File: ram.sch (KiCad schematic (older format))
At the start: 7 parts, among them U1 LFE5U-85F-6BG381C

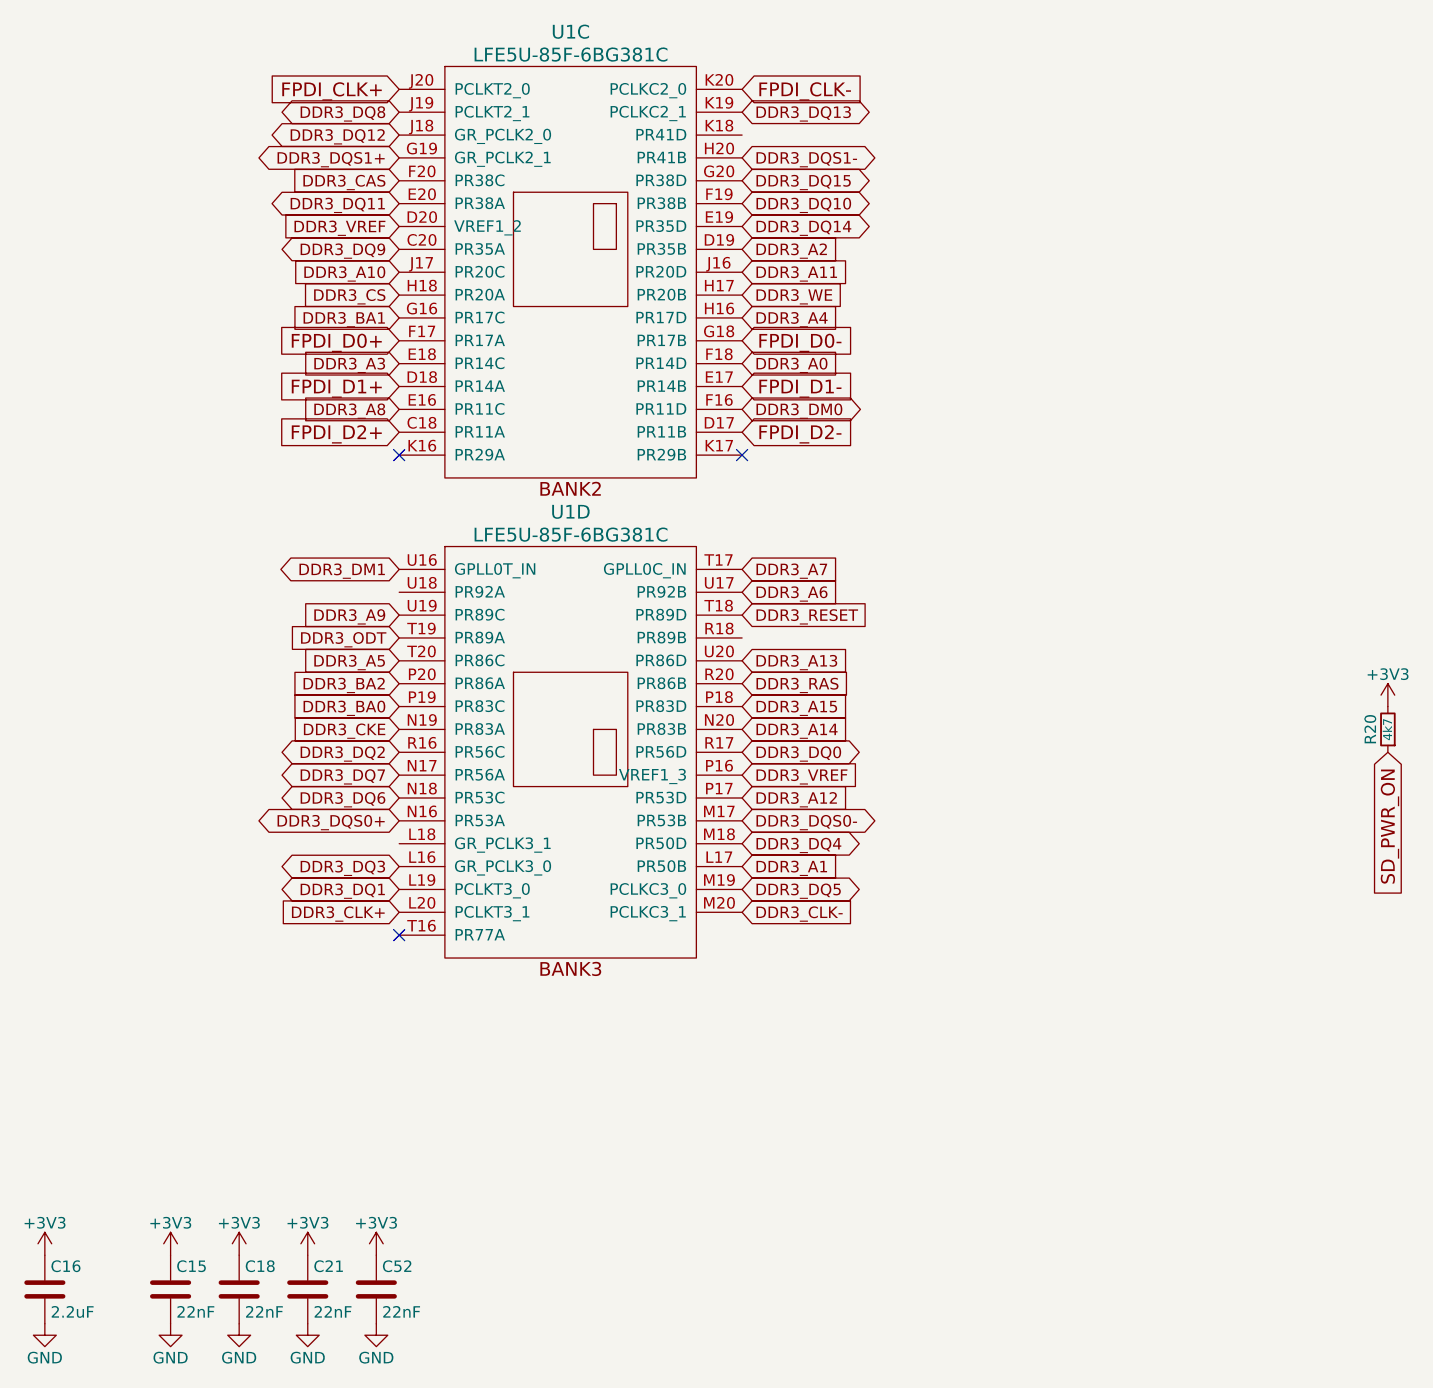
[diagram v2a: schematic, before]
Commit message: Adding SDRAM removind DDR3
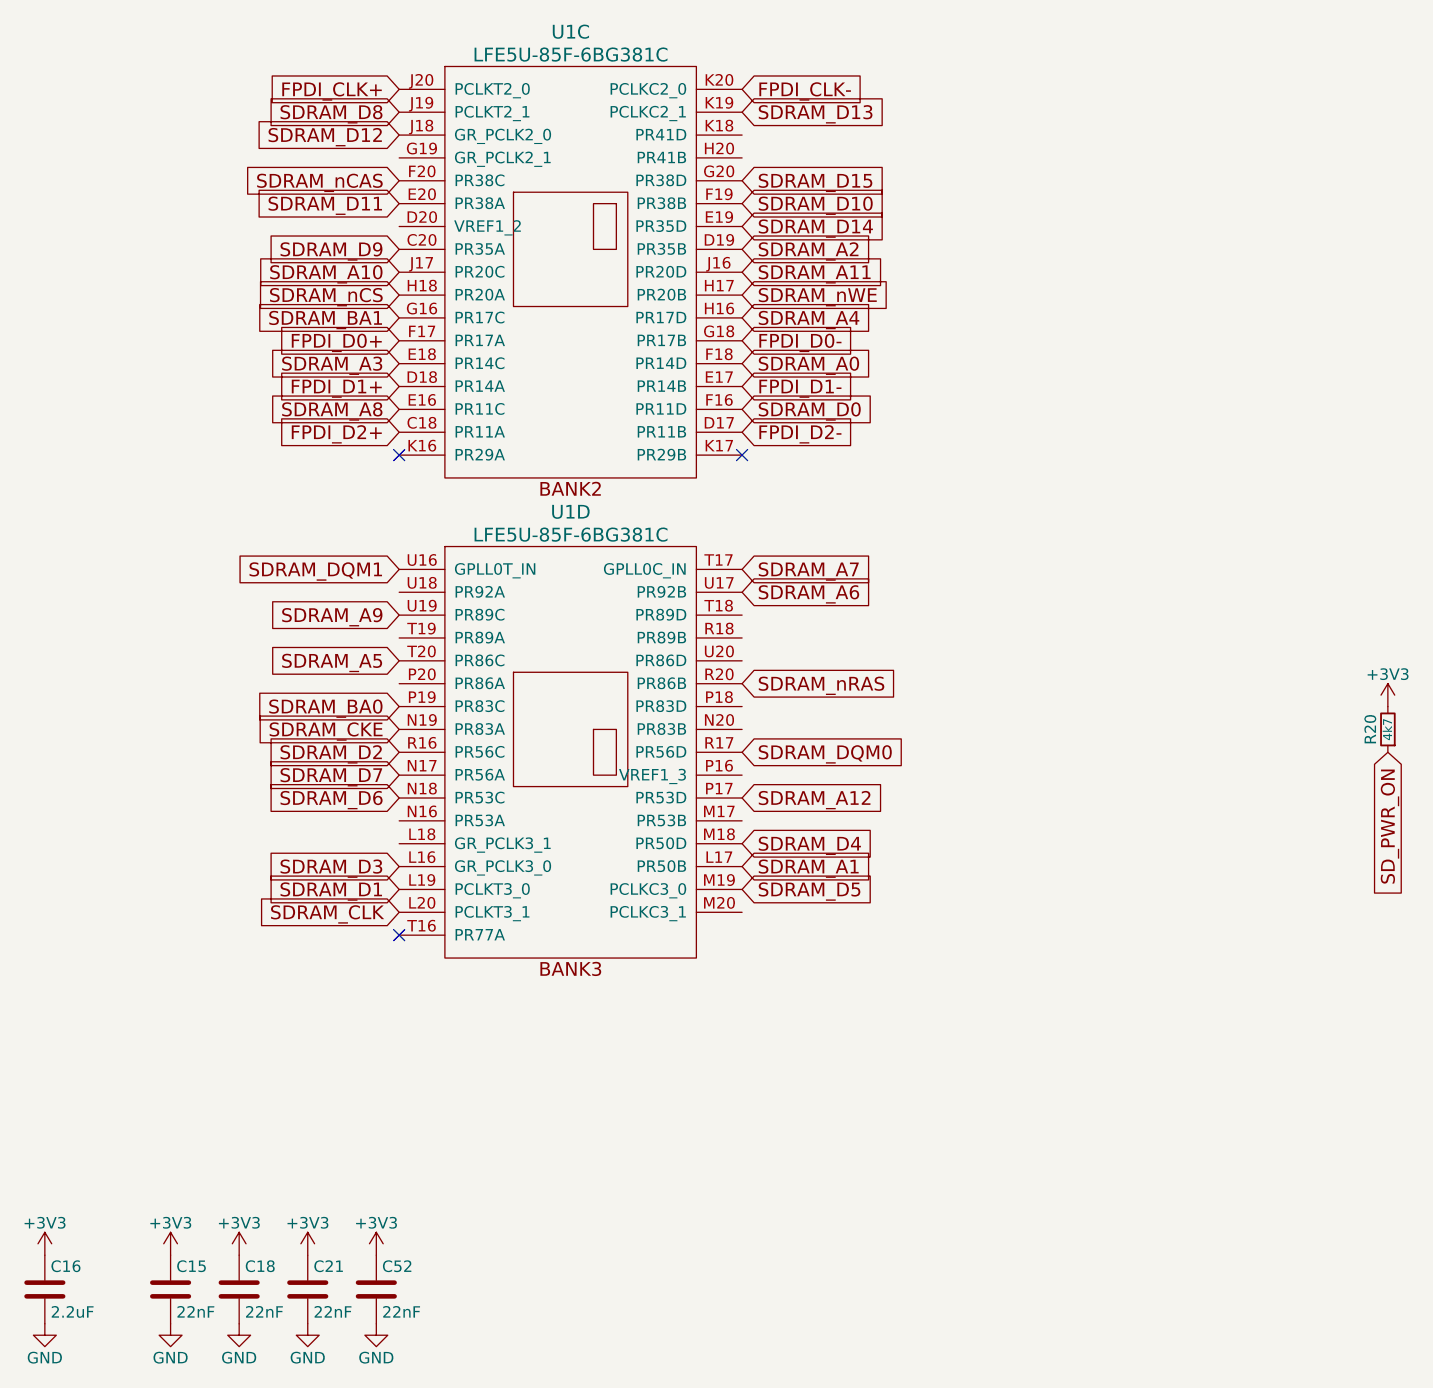
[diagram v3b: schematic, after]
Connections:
- net DDR3_A0 renamed SDRAM_A0
- net DDR3_A1 renamed SDRAM_A1
- net DDR3_A10 renamed SDRAM_A10
- net DDR3_A11 renamed SDRAM_A11
- net DDR3_A12 renamed SDRAM_A12
- net DDR3_A13: no longer names the net of U1.U20 (PR86D)
- net DDR3_A14: no longer names the net of U1.N20 (PR83B)
- net DDR3_A15: no longer names the net of U1.P18 (PR83D)
- net DDR3_A2 renamed SDRAM_A2
- net DDR3_A3 renamed SDRAM_A3
- net DDR3_A4 renamed SDRAM_A4
- net DDR3_A5 renamed SDRAM_A5
- net DDR3_A6 renamed SDRAM_A6
- net DDR3_A7 renamed SDRAM_A7
- net DDR3_A8 renamed SDRAM_A8
- net DDR3_A9 renamed SDRAM_A9
- net DDR3_BA0 renamed SDRAM_BA0
- net DDR3_BA1 renamed SDRAM_BA1
- net DDR3_BA2: no longer names the net of U1.P20 (PR86A)
- net DDR3_CAS renamed SDRAM_nCAS
- net DDR3_CKE renamed SDRAM_CKE
- net DDR3_CLK+ renamed SDRAM_CLK
- net DDR3_CLK-: no longer names the net of U1.M20 (PCLKC3_1)
- net DDR3_CS renamed SDRAM_nCS
- net DDR3_DM0 renamed SDRAM_D0
- net DDR3_DM1 renamed SDRAM_DQM1
- net DDR3_DQ0 renamed SDRAM_DQM0
- net DDR3_DQ1 renamed SDRAM_D1
- net DDR3_DQ10 renamed SDRAM_D10
- net DDR3_DQ11 renamed SDRAM_D11
- net DDR3_DQ12 renamed SDRAM_D12
- net DDR3_DQ13 renamed SDRAM_D13
- net DDR3_DQ14 renamed SDRAM_D14
- net DDR3_DQ15 renamed SDRAM_D15
- net DDR3_DQ2 renamed SDRAM_D2
- net DDR3_DQ3 renamed SDRAM_D3
- net DDR3_DQ4 renamed SDRAM_D4
- net DDR3_DQ5 renamed SDRAM_D5
- net DDR3_DQ6 renamed SDRAM_D6
- net DDR3_DQ7 renamed SDRAM_D7
- net DDR3_DQ8 renamed SDRAM_D8
- net DDR3_DQ9 renamed SDRAM_D9
- net DDR3_DQS0+: no longer names the net of U1.N16 (PR53A)
- net DDR3_DQS0-: no longer names the net of U1.M17 (PR53B)
- net DDR3_DQS1+: no longer names the net of U1.G19 (GR_PCLK2_1)
- net DDR3_DQS1-: no longer names the net of U1.H20 (PR41B)
- net DDR3_ODT: no longer names the net of U1.T19 (PR89A)
- net DDR3_RAS renamed SDRAM_nRAS
- net DDR3_RESET: no longer names the net of U1.T18 (PR89D)
- net DDR3_VREF: no longer names the net of U1.D20 (VREF1_2)
- net DDR3_VREF: no longer U1.P16 (VREF1_3)
- net DDR3_WE renamed SDRAM_nWE
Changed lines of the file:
@@
 	-1   0    0    1
 $EndComp
-Text GLabel 8100 5100 2    50   Input ~ 0
-DDR3_A1
-Text GLabel 8100 2400 2    50   Input ~ 0
-DDR3_A2
-Text GLabel 6600 2900 0    50   Input ~ 0
-DDR3_A3
-Text GLabel 8100 2700 2    50   Input ~ 0
-DDR3_A4
-Text GLabel 8100 3900 2    50   Input ~ 0
-DDR3_A6
-Text GLabel 8100 3800 2    50   Input ~ 0
-DDR3_A7
-Text GLabel 6600 3100 0    50   Input ~ 0
-DDR3_A8
-Text GLabel 6600 4000 0    50   Input ~ 0
-DDR3_A9
-Text GLabel 6600 2500 0    50   Input ~ 0
-DDR3_A10
-Text GLabel 8100 2500 2    50   Input ~ 0
-DDR3_A11
-Text GLabel 8100 4800 2    50   Input ~ 0
-DDR3_A12
-Text GLabel 8100 4500 2    50   Input ~ 0
-DDR3_A14
-Text GLabel 6600 4400 0    50   Input ~ 0
-DDR3_BA0
-Text GLabel 6600 2700 0    50   Input ~ 0
-DDR3_BA1
-Text GLabel 6600 4300 0    50   Input ~ 0
-DDR3_BA2
-Text GLabel 6600 5300 0    50   Input ~ 0
-DDR3_CLK+
-Text GLabel 8100 5300 2    50   Input ~ 0
-DDR3_CLK-
-Text GLabel 6600 4500 0    50   Input ~ 0
-DDR3_CKE
-Text GLabel 8100 4000 2    50   Input ~ 0
-DDR3_RESET
-Text GLabel 6600 2600 0    50   Input ~ 0
-DDR3_CS
-Text GLabel 6600 2100 0    50   Input ~ 0
-DDR3_CAS
-Text GLabel 8100 4300 2    50   Input ~ 0
-DDR3_RAS
-Text GLabel 8100 2600 2    50   Input ~ 0
-DDR3_WE
-Text GLabel 6600 4100 0    50   Input ~ 0
-DDR3_ODT
-Text GLabel 8100 4600 2    50   BiDi ~ 0
-DDR3_DQ0
-Text GLabel 6600 5200 0    50   BiDi ~ 0
-DDR3_DQ1
-Text GLabel 6600 4600 0    50   BiDi ~ 0
-DDR3_DQ2
-Text GLabel 6600 5100 0    50   BiDi ~ 0
-DDR3_DQ3
-Text GLabel 8100 5000 2    50   BiDi ~ 0
-DDR3_DQ4
-Text GLabel 8100 5200 2    50   BiDi ~ 0
-DDR3_DQ5
-Text GLabel 6600 4800 0    50   BiDi ~ 0
-DDR3_DQ6
-Text GLabel 6600 4700 0    50   BiDi ~ 0
-DDR3_DQ7
-Text GLabel 8100 2200 2    50   BiDi ~ 0
-DDR3_DQ10
-Text GLabel 6600 2200 0    50   BiDi ~ 0
-DDR3_DQ11
-Text GLabel 6600 1900 0    50   BiDi ~ 0
-DDR3_DQ12
-Text GLabel 8100 2300 2    50   BiDi ~ 0
-DDR3_DQ14
-Text GLabel 8100 2100 2    50   BiDi ~ 0
-DDR3_DQ15
-Text GLabel 6600 3800 0    50   BiDi ~ 0
-DDR3_DM1
-Text GLabel 6600 4900 0    50   BiDi ~ 0
-DDR3_DQS0+
-Text GLabel 8100 4900 2    50   BiDi ~ 0
-DDR3_DQS0-
-Text GLabel 8100 4400 2    50   Input ~ 0
-DDR3_A15
-Text GLabel 6600 4200 0    50   Input ~ 0
-DDR3_A5
-Text GLabel 8100 4200 2    50   Input ~ 0
-DDR3_A13
-Text GLabel 6600 2400 0    50   BiDi ~ 0
-DDR3_DQ9
-Text GLabel 8100 1800 2    50   BiDi ~ 0
-DDR3_DQ13
-Text GLabel 8100 3100 2    50   BiDi ~ 0
-DDR3_DM0
-Text GLabel 6600 2300 0    50   Input ~ 0
-DDR3_VREF
-Text GLabel 8100 4700 2    50   Input ~ 0
-DDR3_VREF
-Text GLabel 6600 1800 0    50   BiDi ~ 0
-DDR3_DQ8
-Text GLabel 8100 2900 2    50   Input ~ 0
-DDR3_A0
-Text GLabel 6600 2000 0    50   BiDi ~ 0
-DDR3_DQS1+
-Text GLabel 8100 2000 2    50   BiDi ~ 0
-DDR3_DQS1-
+Text GLabel 8100 4800 2    60   Input ~ 0
+SDRAM_A12
+Text GLabel 6600 2600 0    60   Input ~ 0
+SDRAM_nCS
+Text GLabel 8100 2600 2    60   Input ~ 0
+SDRAM_nWE
+Text GLabel 6600 2100 0    60   Input ~ 0
+SDRAM_nCAS
+Text GLabel 8100 4300 2    60   Input ~ 0
+SDRAM_nRAS
+Text GLabel 6600 4500 0    60   Input ~ 0
+SDRAM_CKE
+Text GLabel 6600 5300 0    60   Input ~ 0
+SDRAM_CLK
+Text GLabel 6600 2700 0    60   Input ~ 0
+SDRAM_BA1
+Text GLabel 6600 4400 0    60   Input ~ 0
+SDRAM_BA0
+Text GLabel 8100 2500 2    60   Input ~ 0
+SDRAM_A11
+Text GLabel 6600 2500 0    60   Input ~ 0
+SDRAM_A10
+Text GLabel 6600 4000 0    60   Input ~ 0
+SDRAM_A9
+Text GLabel 6600 3100 0    60   Input ~ 0
+SDRAM_A8
+Text GLabel 8100 3800 2    60   Input ~ 0
+SDRAM_A7
+Text GLabel 8100 3900 2    60   Input ~ 0
+SDRAM_A6
+Text GLabel 6600 4200 0    60   Input ~ 0
+SDRAM_A5
+Text GLabel 8100 2700 2    60   Input ~ 0
+SDRAM_A4
+Text GLabel 6600 2900 0    60   Input ~ 0
+SDRAM_A3
+Text GLabel 8100 2400 2    60   Input ~ 0
+SDRAM_A2
+Text GLabel 8100 5100 2    60   Input ~ 0
+SDRAM_A1
+Text GLabel 8100 2900 2    60   Input ~ 0
+SDRAM_A0
+Text GLabel 6600 3800 0    60   Input ~ 0
+SDRAM_DQM1
+Text GLabel 8100 4600 2    60   Input ~ 0
+SDRAM_DQM0
+Text GLabel 8100 2100 2    60   Input ~ 0
+SDRAM_D15
+Text GLabel 8100 2300 2    60   Input ~ 0
+SDRAM_D14
+Text GLabel 8100 1800 2    60   Input ~ 0
+SDRAM_D13
+Text GLabel 6600 1900 0    60   Input ~ 0
+SDRAM_D12
+Text GLabel 6600 2200 0    60   Input ~ 0
+SDRAM_D11
+Text GLabel 8100 2200 2    60   Input ~ 0
+SDRAM_D10
+Text GLabel 6600 2400 0    60   Input ~ 0
+SDRAM_D9
+Text GLabel 6600 1800 0    60   Input ~ 0
+SDRAM_D8
+Text GLabel 6600 4700 0    60   Input ~ 0
+SDRAM_D7
+Text GLabel 6600 4800 0    60   Input ~ 0
+SDRAM_D6
+Text GLabel 8100 5200 2    60   Input ~ 0
+SDRAM_D5
+Text GLabel 8100 5000 2    60   Input ~ 0
+SDRAM_D4
+Text GLabel 6600 5100 0    60   Input ~ 0
+SDRAM_D3
+Text GLabel 6600 4600 0    60   Input ~ 0
+SDRAM_D2
+Text GLabel 6600 5200 0    60   Input ~ 0
+SDRAM_D1
+Text GLabel 8100 3100 2    60   Input ~ 0
+SDRAM_D0
 $EndSCHEMATC
